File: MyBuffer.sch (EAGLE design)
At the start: 102 parts, among them Q1 BD140, Q2 BD139, Q3 BD140, Q4 BD139, Q5 BD139, Q6 BD139, T10 BD140, T11 BD139, T12 BD140, T13 BD139, T14 BD140, T17 BD139, T18 BD140, T9 BD139

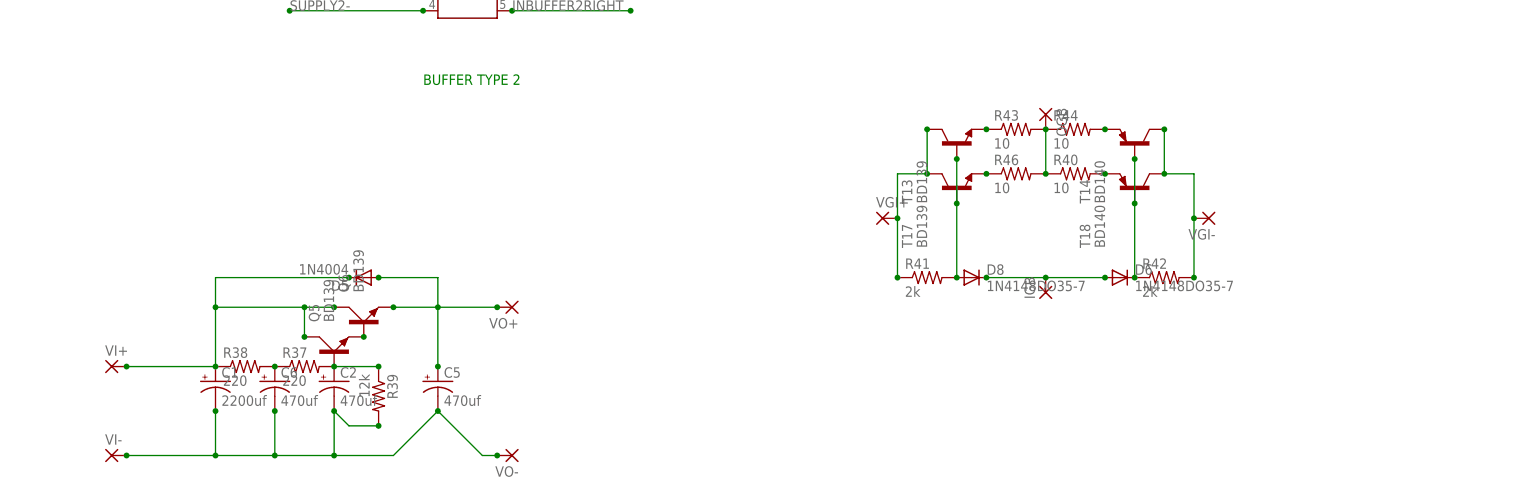
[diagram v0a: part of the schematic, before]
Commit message: Initial Commit
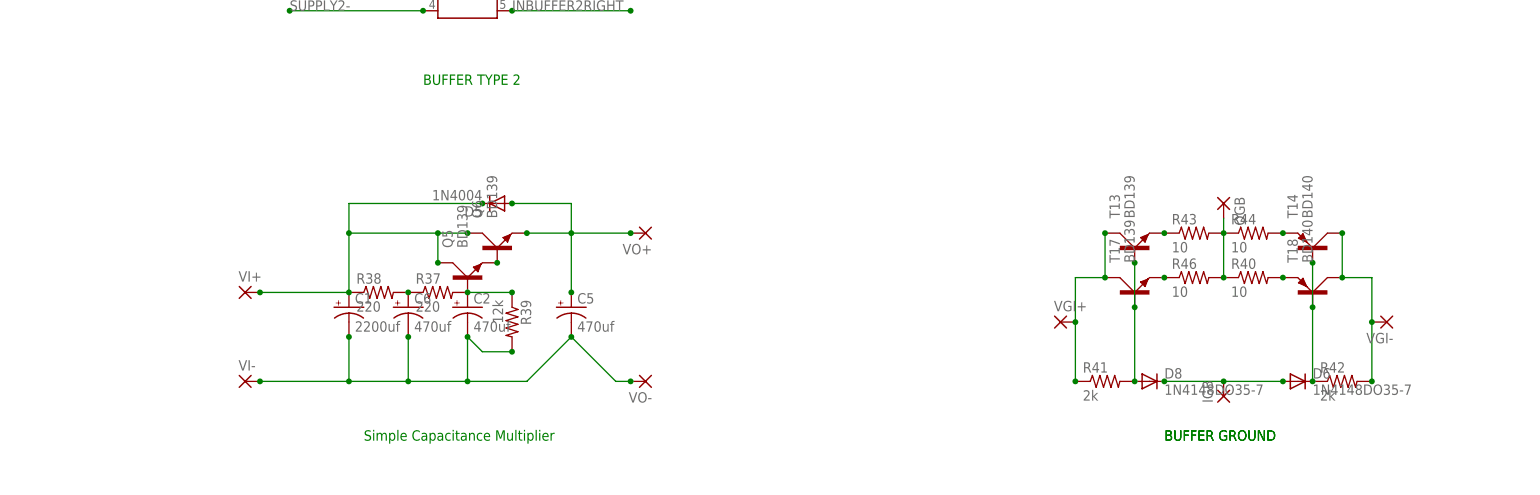
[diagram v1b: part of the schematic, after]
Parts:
- T13, T17: device transistor-npn:BD139 -> transistor-power:BD139
- T14, T18: device transistor-pnp:BD140 -> transistor-power:BD140
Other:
- note added: "BUFFER GROUND"
- note added: "Simple Capacitance Multiplier"
- moved on the sheet: C1, C2, C5, C6, D5, D6, D8, IGB, OGB, Q5, Q6, R37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
